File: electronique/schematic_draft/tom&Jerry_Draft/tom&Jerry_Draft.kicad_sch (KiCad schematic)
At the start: 0 parts

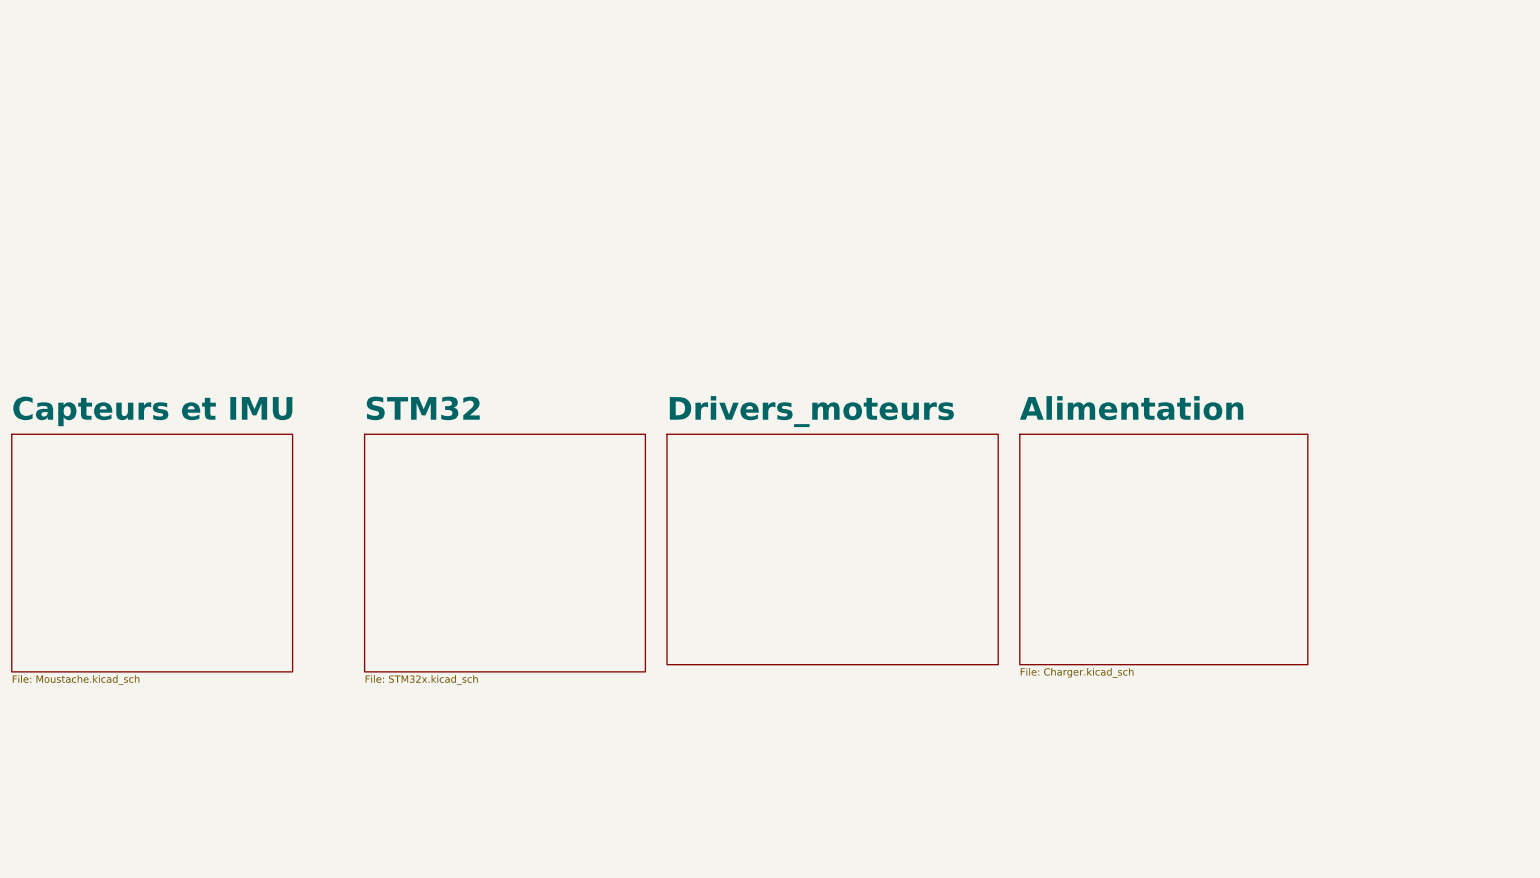
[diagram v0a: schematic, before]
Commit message: STM32 KiCAD V2 - 18.09.2024
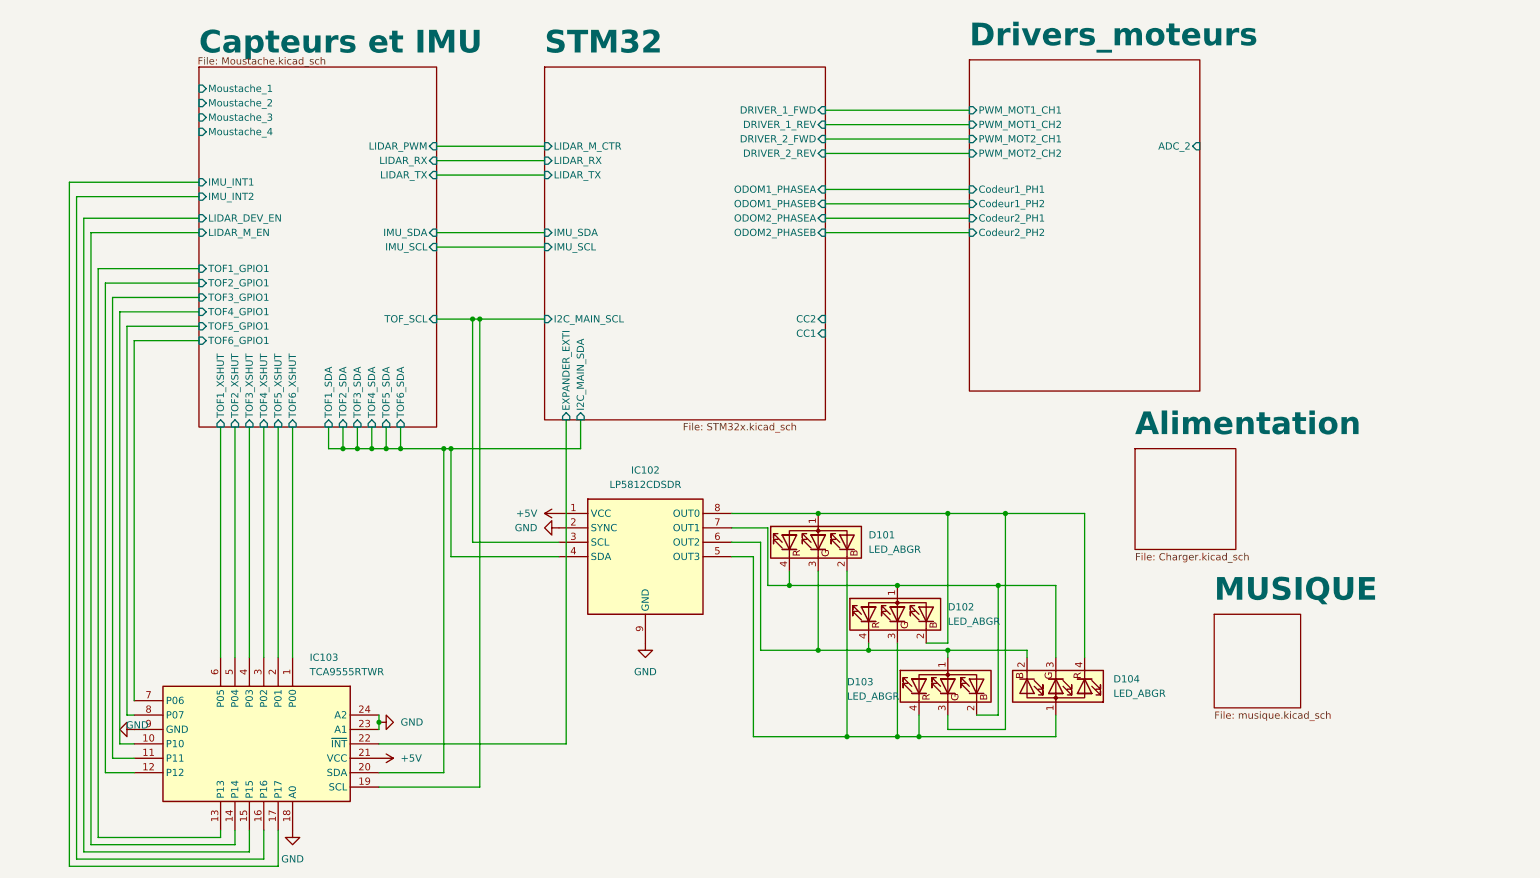
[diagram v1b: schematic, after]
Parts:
- added D101, D102, D103, D104: LED_ABGR, symbol Device:LED_ABGR
- added IC102: LP5812CDSDR, SON65P300X300X80-9N-D, symbol LP5812CDSDR:LP5812CDSDR
- added IC103: TCA9555RTWR, QFN50P400X400X80-25N-D, symbol TCA9555RTWR:TCA9555RTWR
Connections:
- new net: D101.3 (GK), D102.4 (RK), D103.1 (A), D104.2 (BK), IC102.6 (OUT2)
- new net: D101.4 (RK), D102.1 (A), D103.2 (BK), D104.3 (GK), IC102.7 (OUT1)
- new net: D101.1 (A), D102.2 (BK), D103.3 (GK), D104.4 (RK), IC102.8 (OUT0)
- new net: D101.2 (BK), D102.3 (GK), D103.4 (RK), D104.1 (A), IC102.5 (OUT3)
- new net +5V: IC102.1 (VCC), IC103.21 (VCC)
- new net Capteurs et IMU/IMU_INT1: IC103.17 (P17)
- new net Capteurs et IMU/IMU_INT2: IC103.16 (P16)
- new net Capteurs et IMU/LIDAR_DEV_EN: IC103.15 (P15)
- new net Capteurs et IMU/LIDAR_M_EN: IC103.14 (P14)
- new net Capteurs et IMU/TOF1_GPIO1: IC103.13 (P13)
- new net Capteurs et IMU/TOF1_SDA: IC102.4 (SDA), IC103.20 (SDA)
- new net Capteurs et IMU/TOF1_XSHUT: IC103.6 (P05)
- new net Capteurs et IMU/TOF2_GPIO1: IC103.12 (P12)
- new net Capteurs et IMU/TOF2_XSHUT: IC103.5 (P04)
- new net Capteurs et IMU/TOF3_GPIO1: IC103.11 (P11)
- new net Capteurs et IMU/TOF3_XSHUT: IC103.4 (P03)
- new net Capteurs et IMU/TOF4_GPIO1: IC103.10 (P10)
- new net Capteurs et IMU/TOF4_XSHUT: IC103.3 (P02)
- new net Capteurs et IMU/TOF5_GPIO1: IC103.8 (P07)
- new net Capteurs et IMU/TOF5_XSHUT: IC103.2 (P01)
- new net Capteurs et IMU/TOF6_GPIO1: IC103.7 (P06)
- new net Capteurs et IMU/TOF6_XSHUT: IC103.1 (P00)
- new net Capteurs et IMU/TOF_SCL: IC102.3 (SCL), IC103.19 (SCL)
- new net GND: IC102.2 (SYNC), IC102.9 (GND), IC103.18 (A0), IC103.23 (A1), IC103.24 (A2), IC103.9 (GND)
- new net STM32/EXPANDER_EXTI: IC103.22 (~{INT})
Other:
- added sheet MUSIQUE (musique.kicad_sch)
- sheet Capteurs et IMU ports: added IMU_INT1, IMU_INT2, IMU_SCL, IMU_SDA, LIDAR_DEV_EN, LIDAR_M_EN, LIDAR_PWM, LIDAR_RX, LIDAR_TX, Moustache_1, Moustache_2, Moustache_3, Moustache_4, TOF1_GPIO1, TOF1_SDA, TOF1_XSHUT, TOF2_GPIO1, TOF2_SDA, TOF2_XSHUT, TOF3_GPIO1, TOF3_SDA, TOF3_XSHUT, TOF4_GPIO1, TOF4_SDA, TOF4_XSHUT, TOF5_GPIO1, TOF5_SDA, TOF5_XSHUT, TOF6_GPIO1, TOF6_SDA, TOF6_XSHUT, TOF_SCL; removed none
- sheet Drivers_moteurs ports: added ADC_2, Codeur1_PH1, Codeur1_PH2, Codeur2_PH1, Codeur2_PH2, PWM_MOT1_CH1, PWM_MOT1_CH2, PWM_MOT2_CH1, PWM_MOT2_CH2; removed none
- sheet STM32 ports: added CC1, CC2, DRIVER_1_FWD, DRIVER_1_REV, DRIVER_2_FWD, DRIVER_2_REV, EXPANDER_EXTI, I2C_MAIN_SCL, I2C_MAIN_SDA, IMU_SCL, IMU_SDA, LIDAR_M_CTR, LIDAR_RX, LIDAR_TX, ODOM1_PHASEA, ODOM1_PHASEB, ODOM2_PHASEA, ODOM2_PHASEB; removed none

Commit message: KiCAD V3 - 18.09.2024
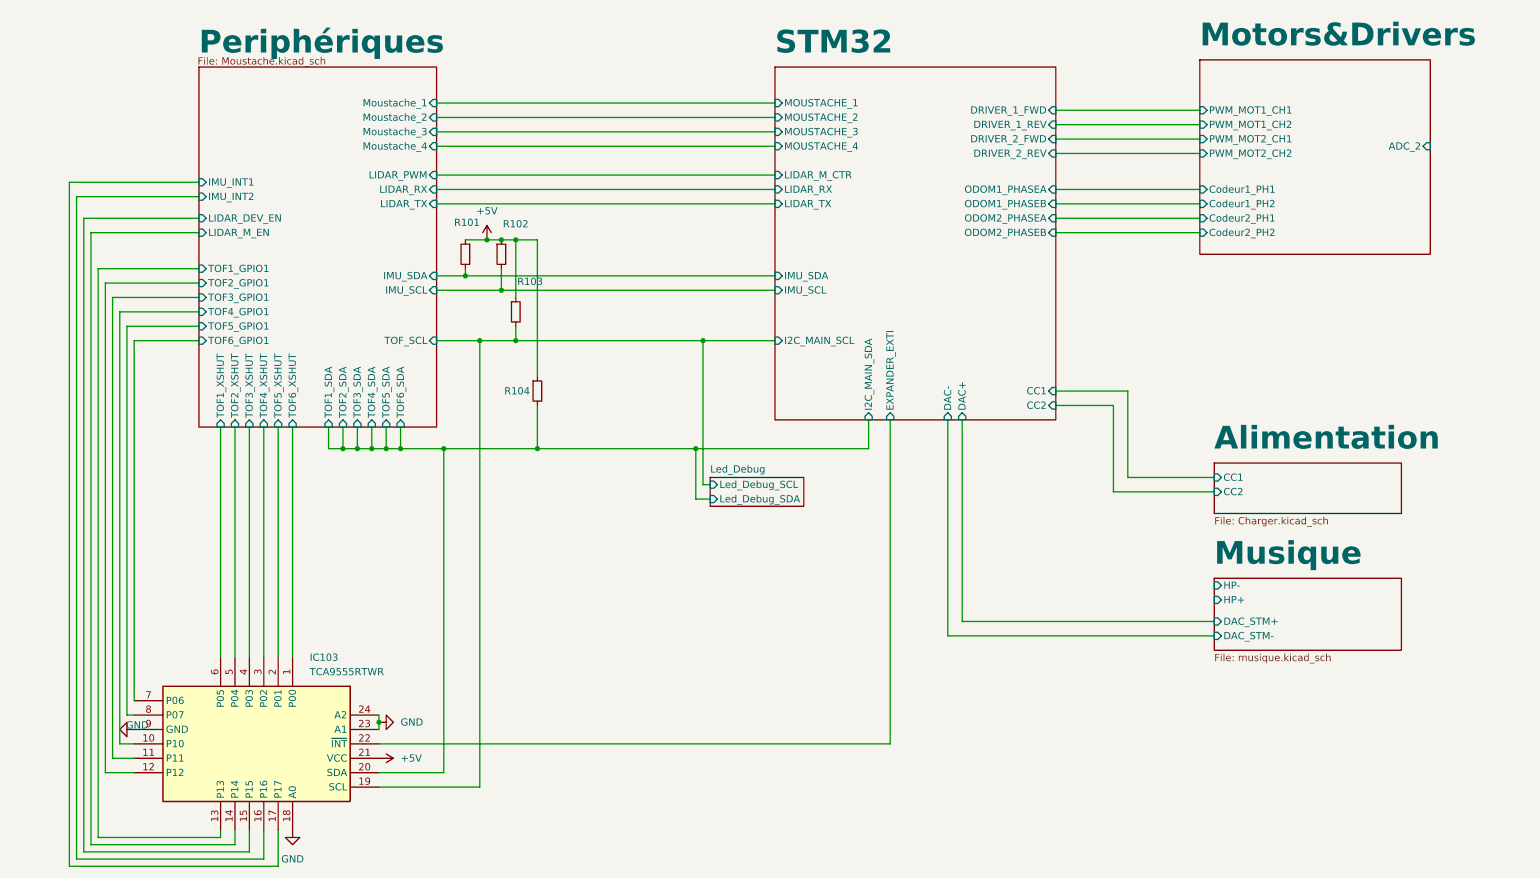
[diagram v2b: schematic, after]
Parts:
- removed D101, D102, D103, D104: LED_ABGR, symbol Device:LED_ABGR
- removed IC102: LP5812CDSDR, SON65P300X300X80-9N-D, symbol LP5812CDSDR:LP5812CDSDR
- added R101, R102, R103, R104: R_Small, symbol Device:R_Small
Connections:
- net +5V: now also R101.1, R102.1, R103.1, R104.1
- net Periphériques/IMU_SCL: now also R102.2
- net Periphériques/IMU_SDA: now also R101.2
- net Periphériques/TOF1_SDA renamed Led_Debug/Led_Debug_SDA
- net Led_Debug/Led_Debug_SDA: now also R104.2
- net Periphériques/TOF_SCL renamed Led_Debug/Led_Debug_SCL
- net Led_Debug/Led_Debug_SCL: now also R103.2
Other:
- sheet Capteurs et IMU renamed Periphériques
- sheet Drivers_moteurs renamed Motors&Drivers
- sheet MUSIQUE renamed Musique
- added sheet Led_Debug (Led_Debug.kicad_sch)
- sheet Alimentation ports: added CC1, CC2; removed none
- sheet Musique ports: added DAC_STM+, DAC_STM-, HP+, HP-; removed none
- sheet STM32 ports: added DAC+, DAC-, MOUSTACHE_1, MOUSTACHE_2, MOUSTACHE_3, MOUSTACHE_4; removed none
